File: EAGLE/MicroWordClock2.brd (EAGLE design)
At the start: 108 x 108 mm, 83 parts, among them J1 DS3231S#T&RMODULE, J2 10118193-0001LF, J3 AVR_SPI_PROG_3X2PTH, U1 ATMEGA328P

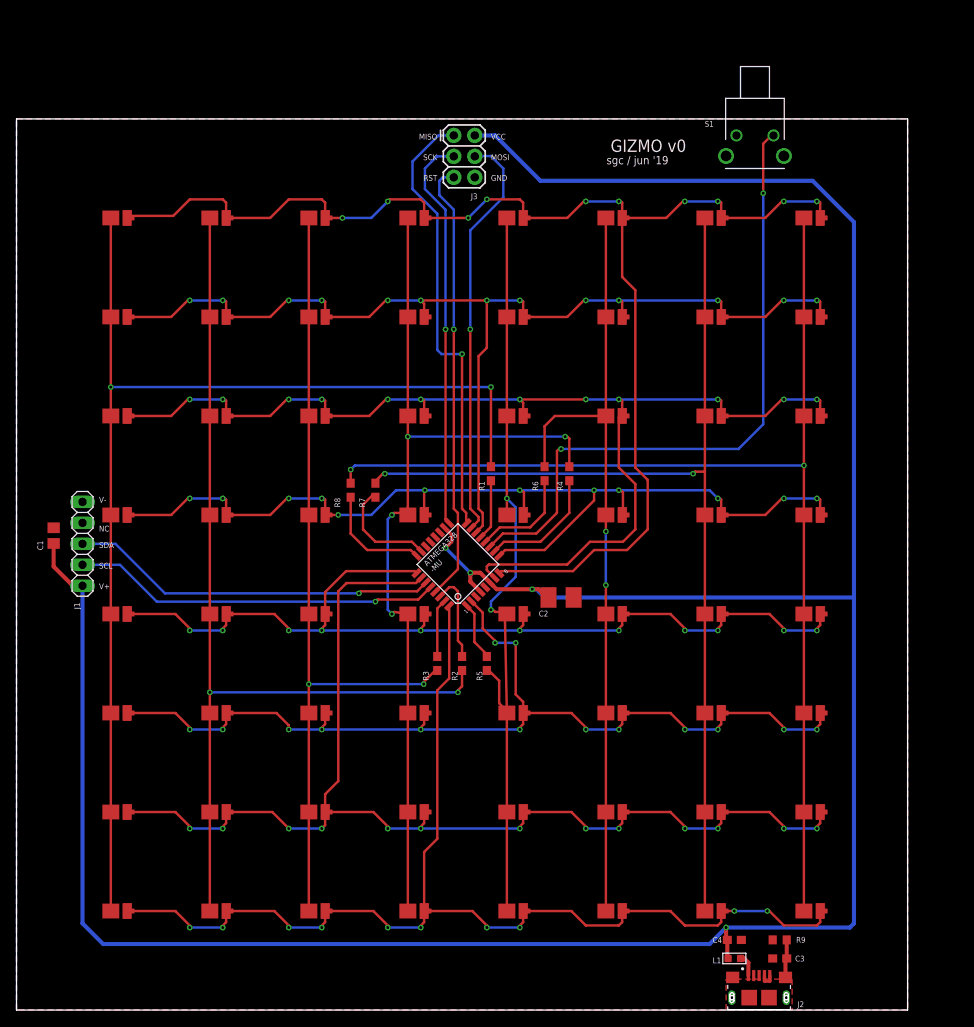
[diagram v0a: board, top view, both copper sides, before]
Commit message: adding the dxf
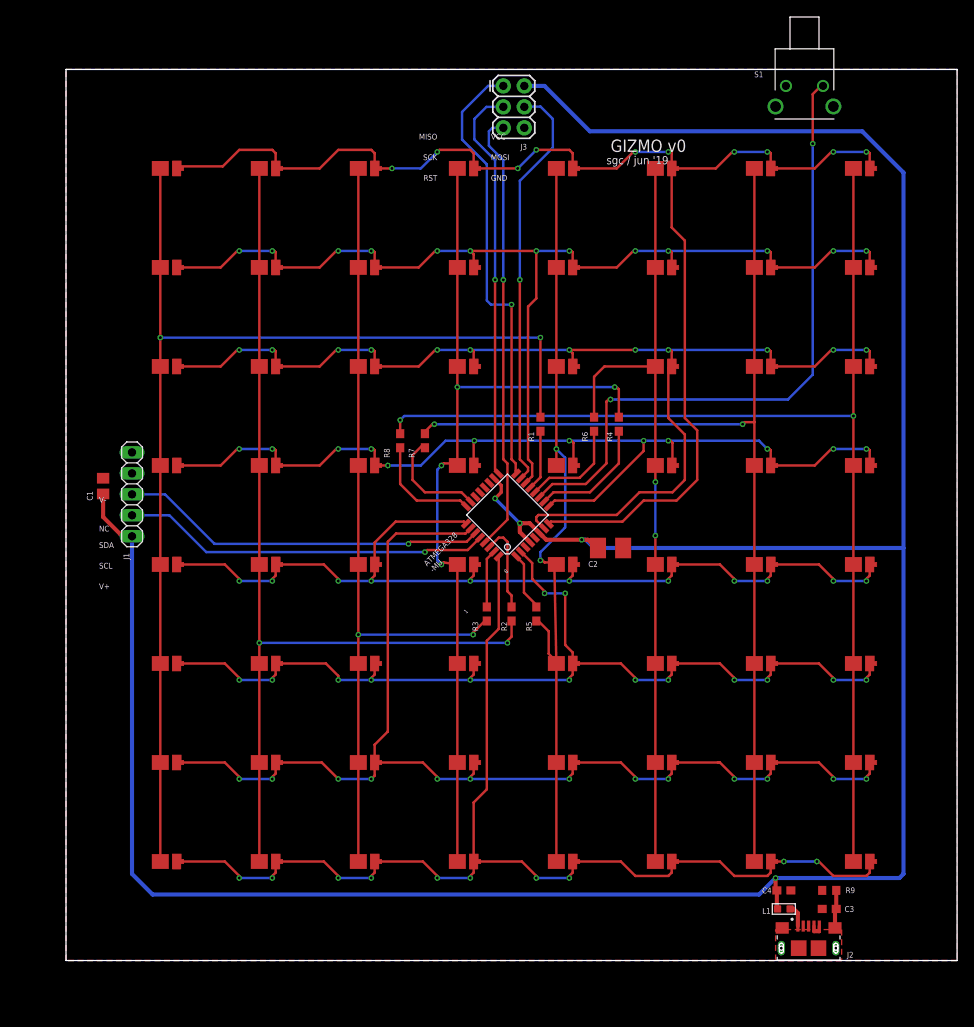
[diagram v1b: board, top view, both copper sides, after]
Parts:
- moved C1 8.49 mm to (10.5, 63.5)
- moved C2 8.49 mm to (72.0, 56.0)
- moved C3 8.49 mm to (98.5, 12.2)
- moved C4 8.49 mm to (93.0, 14.5)
- moved J1 8.49 mm to (14.0, 62.5)
- moved J2 8.49 mm to (96.0, 7.50)
- moved J3 8.49 mm to (59.0, 112.0)
- moved L1 8.49 mm to (93.0, 12.2)
- moved R1 8.49 mm to (63.5, 71.0)
- moved R2 8.49 mm to (60.0, 48.0)
- moved R3 8.49 mm to (57.0, 48.0)
- moved R4 8.49 mm to (73.0, 71.0)
- moved R5 8.49 mm to (63.0, 48.0)
- moved R6 8.49 mm to (70.0, 71.0)
- moved R7 8.49 mm to (49.5, 69.0)
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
